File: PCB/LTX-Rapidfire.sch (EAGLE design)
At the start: 52 parts, among them J1 F-1X08-SIP-100-40Y, Q1 MMBT3904, Q10 SS8550D, Q11 2N3906, Q12 2N3906, Q13 MMBT3904, Q2 2N3906, Q3 MMBT3904, Q4 MMBT3904, Q5 MMBT3904, Q6 2N3906, Q7 2N3906, Q8 2N3906, Q9 MMBT3904, SW1 F-1X02-SIP-100-40, U1 XC6206P332MR, U3 ATTINY1616-MNRVQFN20_3X3_MCH-M

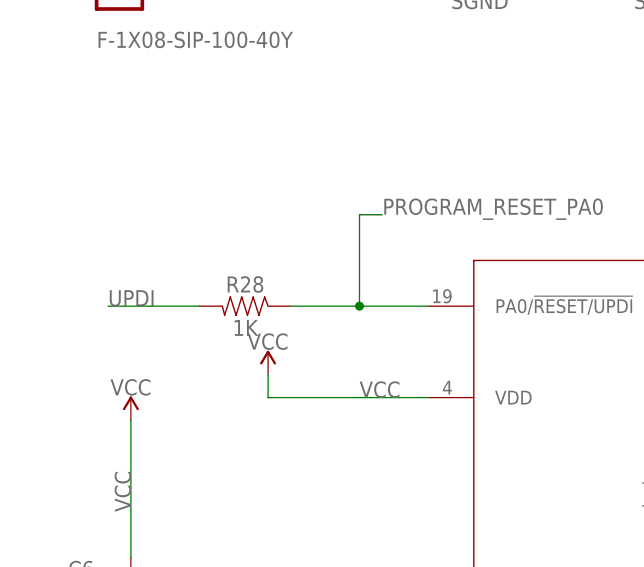
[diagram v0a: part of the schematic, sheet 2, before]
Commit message: Updated gerbers, com, and placement
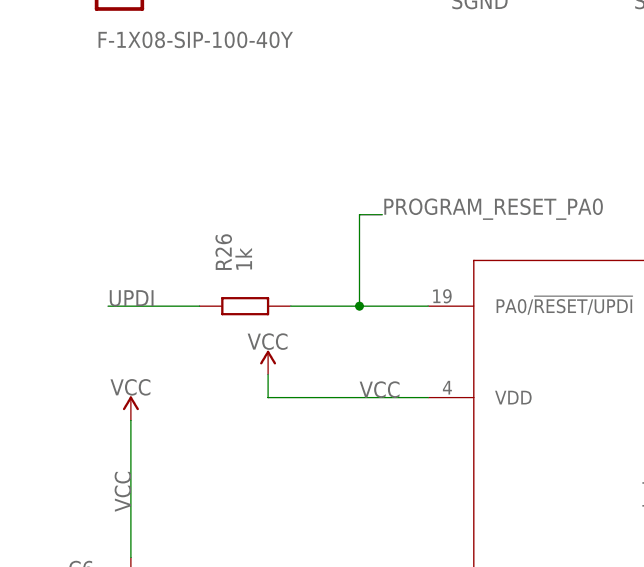
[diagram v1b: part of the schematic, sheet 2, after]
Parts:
- removed R28: 1K, SparkFun-Resistors:2.2KOHM-0402-1/16W-1%
- added R26: 1k, JLC PCB Basic Parts_loc:R_1K_0603
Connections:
- net PROGRAM_RESET_PA0: now also R26.1; no longer R28.1
- net UPDI: now also R26.2; no longer R28.2
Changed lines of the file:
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@@
 <attribute name="LCSC_PART" value="C66801"/>
 </part>
-<part name="R28" library="SparkFun-Resistors" deviceset="2.2KOHM" device="-0402-1/16W-1%" value="1K"/>
 <part name="SUPPLY10" library="supply2" deviceset="GND" device=""/>
 <part name="SUPPLY2" library="supply2" deviceset="GND" device=""/>
@@
 <part name="SUPPLY16" library="supply2" deviceset="+9V" device=""/>
 <part name="JP1" library="adafruit" deviceset="PINHD-1X3" device=""/>
+<part name="R26" library="JLC PCB Basic Parts_loc" deviceset="R_" device="_0603" technology="1K" value="1k"/>
 </parts>
 <sheets>
@@
 </plain>
 <instances>
-<instance part="R28" gate="G$1" x="35.56" y="93.98" rot="MR0"/>
 <instance part="SUPPLY10" gate="GND" x="22.86" y="53.34" rot="MR0"/>
 <instance part="SUPPLY2" gate="GND" x="38.1" y="35.56" rot="MR0"/>
@@
 <instance part="SUPPLY16" gate="G$1" x="58.42" y="157.48"/>
 <instance part="JP1" gate="A" x="226.06" y="144.78"/>
+<instance part="R26" gate="R1" x="35.56" y="93.98" smashed="yes" rot="R180">
+<attribute name="NAME" x="34.0614" y="97.79" size="1.778" layer="95" rot="R90"/>
+<attribute name="VALUE" x="36.322" y="97.79" size="1.778" layer="96" rot="R90"/>
+</instance>
 </instances>
 <busses>
@@
 <net name="UPDI" class="0">
 <segment>
-<pinref part="R28" gate="G$1" pin="2"/>
 <wire x1="30.48" y1="93.98" x2="20.32" y2="93.98" width="0.1524" layer="91"/>
 <label x="20.32" y="93.98" size="1.778" layer="95"/>
+<pinref part="R26" gate="R1" pin="2"/>
 </segment>
 <segment>
@@
 <net name="PROGRAM_RESET_PA0" class="0">
 <segment>
-<pinref part="R28" gate="G$1" pin="1"/>
 <wire x1="40.64" y1="93.98" x2="48.26" y2="93.98" width="0.1524" layer="91"/>
 <pinref part="U3" gate="A" pin="PA0/!RESET/UPDI"/>
@@
 <wire x1="48.26" y1="104.14" x2="50.8" y2="104.14" width="0.1524" layer="91"/>
 <label x="50.8" y="104.14" size="1.778" layer="95"/>
-</segment>
-</net>
+<pinref part="R26" gate="R1" pin="1"/>
+</segment>
+</net>
